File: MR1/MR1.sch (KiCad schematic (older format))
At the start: 16 parts, among them J1 Conn_01x04_Male, J2 Conn_01x04_Male, J3 Conn_01x04_Male, J4 Conn_01x04_Male, J5 Conn_01x02_Male, J6 Conn_01x04_Male, J7 Conn_01x04_Male, J8 Conn_01x04_Male, Q1 2SC1815, U5 LPC1768, U6 MPU6050, U7 R3008SB, U8 MCP2561-E-P

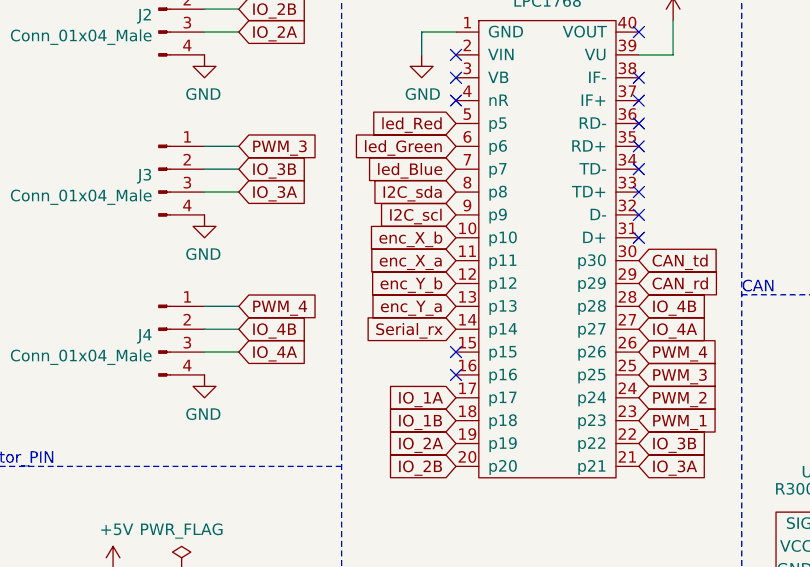
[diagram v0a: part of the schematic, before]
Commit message: fix: MR1
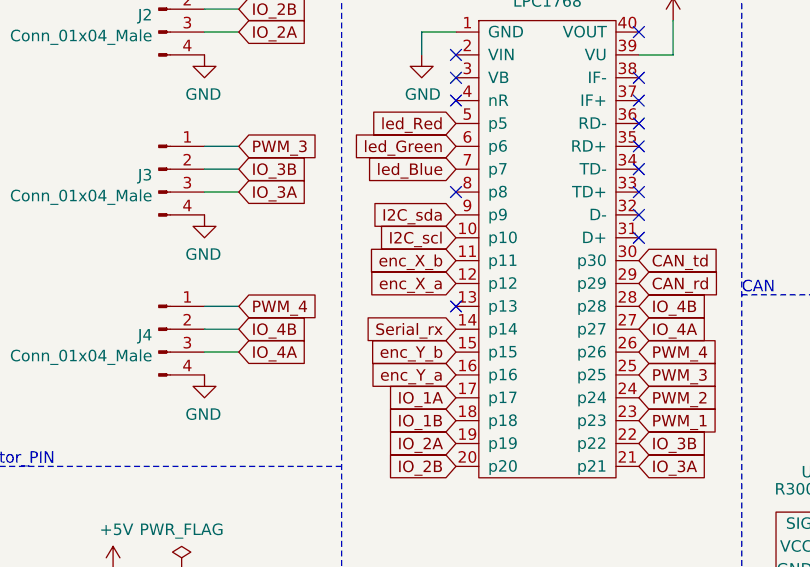
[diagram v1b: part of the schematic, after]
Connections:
- net I2C_scl: now also U5.10 (p10); no longer U5.9 (p9)
- net I2C_sda: now also U5.9 (p9); no longer U5.8 (p8)
- net enc_X_a: now also U5.12 (p12); no longer U5.11 (p11)
- net enc_X_b: now also U5.11 (p11); no longer U5.10 (p10)
- net enc_Y_a: now also U5.16 (p16); no longer U5.13 (p13)
- net enc_Y_b: now also U5.15 (p15); no longer U5.12 (p12)
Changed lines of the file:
@@
 Text GLabel 5300 4350 0    50   Input ~ 0
 Serial_rx
+Text GLabel 5300 3950 0    50   Input ~ 0
+I2C_scl
 Text GLabel 5300 3850 0    50   Input ~ 0
-I2C_scl
-Text GLabel 5300 3750 0    50   Input ~ 0
 I2C_sda
 Text GLabel 5300 4650 0    50   Input ~ 0
@@
 NoConn ~ 6100 3850
 NoConn ~ 6100 3950
-NoConn ~ 5300 4450
-NoConn ~ 5300 4550
 NoConn ~ 5300 3250
 NoConn ~ 5300 3350
@@
 Text Notes 3200 4950 0    50   ~ 0
 Motor_PIN
-Text GLabel 5300 4250 0    50   Input ~ 0
+Text GLabel 5300 4550 0    50   Input ~ 0
 enc_Y_a
-Text GLabel 5300 4050 0    50   Input ~ 0
-enc_X_a
-Text GLabel 5300 3950 0    50   Input ~ 0
-enc_X_b
 Text GLabel 2600 3250 2    50   Input ~ 0
 enc_Y_b
@@
 	1    0    0    -1
 $EndComp
-Text GLabel 5300 4150 0    50   Input ~ 0
+Text GLabel 5300 4450 0    50   Input ~ 0
 enc_Y_b
 Wire Notes Line
@@
 tape_led
 NoConn ~ 2450 5550
+NoConn ~ 5300 4250
+Text GLabel 5300 4050 0    50   Input ~ 0
+enc_X_b
+Text GLabel 5300 4150 0    50   Input ~ 0
+enc_X_a
+NoConn ~ 5300 3750
 $EndSCHEMATC
